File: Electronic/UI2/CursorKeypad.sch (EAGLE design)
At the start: 22 parts, among them IC1 74HCT14N

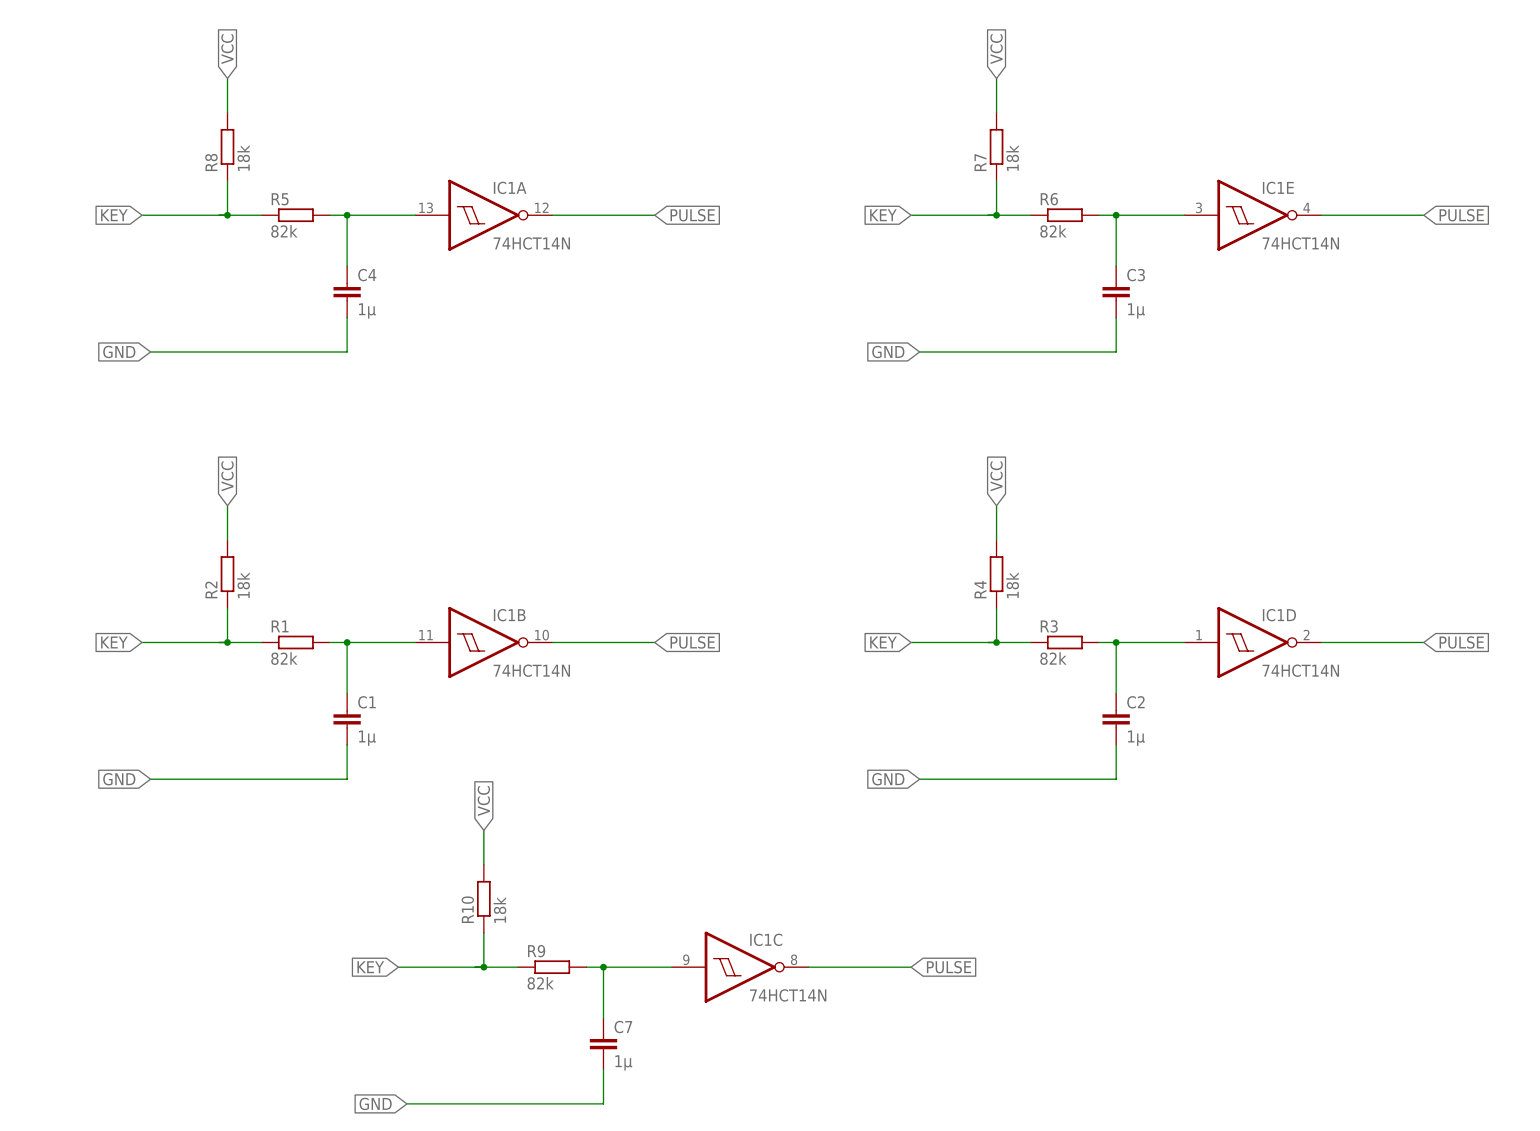
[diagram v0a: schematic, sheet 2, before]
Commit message: new UI
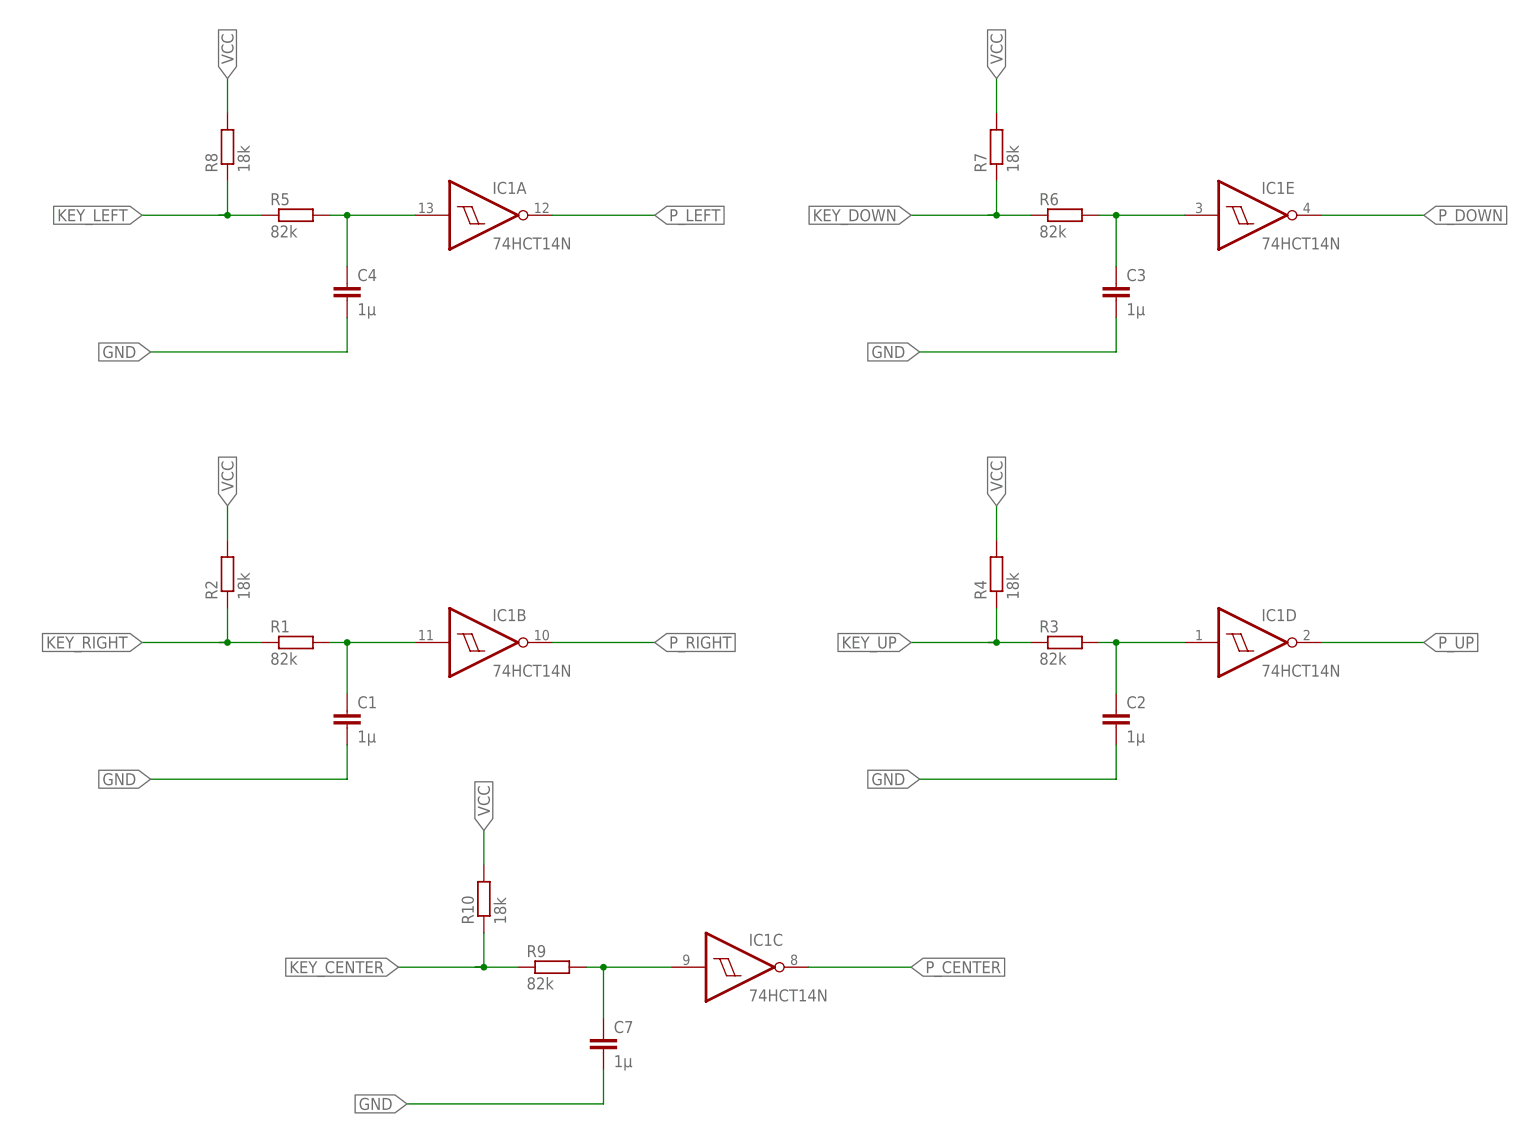
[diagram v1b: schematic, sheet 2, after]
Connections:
- removed net KEY: R1.1, R10.1, R2.1, R3.1, R4.1, R5.1, R6.1, R7.1, R8.1, R9.1
- removed net PULSE: IC1A.O, IC1B.O, IC1C.O, IC1D.O, IC1E.O
- new net P_CENTER: IC1C.O
- new net P_DOWN: IC1E.O
- new net P_LEFT: IC1A.O
- new net P_RIGHT: IC1B.O
- new net P_UP: IC1D.O
- net KEY_CENTER: now also R10.1, R9.1
- net KEY_DOWN: now also R6.1, R7.1
- net KEY_LEFT: now also R5.1, R8.1
- net KEY_RIGHT: now also R1.1, R2.1
- net KEY_UP: now also R3.1, R4.1
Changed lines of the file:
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@@
 </segment>
 </net>
-<net name="PULSE" class="0">
-<segment>
-<wire x1="91.44" y1="139.7" x2="106.68" y2="139.7" width="0.1524" layer="91"/>
-<label x="106.68" y="139.7" size="1.778" layer="95" xref="yes"/>
-<pinref part="IC1" gate="A" pin="O"/>
-</segment>
-<segment>
-<wire x1="91.44" y1="76.2" x2="106.68" y2="76.2" width="0.1524" layer="91"/>
-<label x="106.68" y="76.2" size="1.778" layer="95" xref="yes"/>
-<pinref part="IC1" gate="B" pin="O"/>
-</segment>
-<segment>
-<wire x1="205.74" y1="76.2" x2="220.98" y2="76.2" width="0.1524" layer="91"/>
-<label x="220.98" y="76.2" size="1.778" layer="95" xref="yes"/>
-<pinref part="IC1" gate="D" pin="O"/>
-</segment>
+<net name="P_DOWN" class="0">
 <segment>
 <wire x1="205.74" y1="139.7" x2="220.98" y2="139.7" width="0.1524" layer="91"/>
 <label x="220.98" y="139.7" size="1.778" layer="95" xref="yes"/>
 <pinref part="IC1" gate="E" pin="O"/>
-</segment>
-<segment>
-<wire x1="129.54" y1="27.94" x2="144.78" y2="27.94" width="0.1524" layer="91"/>
-<label x="144.78" y="27.94" size="1.778" layer="95" xref="yes"/>
-<pinref part="IC1" gate="C" pin="O"/>
 </segment>
 </net>
@@
 </segment>
 </net>
-<net name="KEY" class="0">
-<segment>
-<wire x1="43.18" y1="139.7" x2="30.48" y2="139.7" width="0.1524" layer="91"/>
-<wire x1="41.91" y1="139.7" x2="43.18" y2="139.7" width="0.1524" layer="91"/>
-<pinref part="R5" gate="G$1" pin="1"/>
-<pinref part="R8" gate="G$1" pin="1"/>
-<wire x1="43.18" y1="139.7" x2="48.26" y2="139.7" width="0.1524" layer="91"/>
-<wire x1="43.18" y1="144.78" x2="43.18" y2="139.7" width="0.1524" layer="91"/>
-<junction x="43.18" y="139.7"/>
-<label x="30.48" y="139.7" size="1.778" layer="95" rot="R180" xref="yes"/>
-</segment>
-<segment>
-<wire x1="43.18" y1="76.2" x2="30.48" y2="76.2" width="0.1524" layer="91"/>
-<wire x1="41.91" y1="76.2" x2="43.18" y2="76.2" width="0.1524" layer="91"/>
-<pinref part="R1" gate="G$1" pin="1"/>
-<pinref part="R2" gate="G$1" pin="1"/>
-<wire x1="43.18" y1="76.2" x2="48.26" y2="76.2" width="0.1524" layer="91"/>
-<wire x1="43.18" y1="81.28" x2="43.18" y2="76.2" width="0.1524" layer="91"/>
-<junction x="43.18" y="76.2"/>
-<label x="30.48" y="76.2" size="1.778" layer="95" rot="R180" xref="yes"/>
-</segment>
-<segment>
-<wire x1="157.48" y1="76.2" x2="144.78" y2="76.2" width="0.1524" layer="91"/>
-<wire x1="156.21" y1="76.2" x2="157.48" y2="76.2" width="0.1524" layer="91"/>
-<pinref part="R3" gate="G$1" pin="1"/>
-<pinref part="R4" gate="G$1" pin="1"/>
-<wire x1="157.48" y1="76.2" x2="162.56" y2="76.2" width="0.1524" layer="91"/>
-<wire x1="157.48" y1="81.28" x2="157.48" y2="76.2" width="0.1524" layer="91"/>
-<junction x="157.48" y="76.2"/>
-<label x="144.78" y="76.2" size="1.778" layer="95" rot="R180" xref="yes"/>
-</segment>
+<net name="KEY_DOWN" class="0">
 <segment>
 <wire x1="157.48" y1="139.7" x2="144.78" y2="139.7" width="0.1524" layer="91"/>
@@
 <junction x="157.48" y="139.7"/>
 <label x="144.78" y="139.7" size="1.778" layer="95" rot="R180" xref="yes"/>
-</segment>
-<segment>
-<wire x1="81.28" y1="27.94" x2="68.58" y2="27.94" width="0.1524" layer="91"/>
-<wire x1="80.01" y1="27.94" x2="81.28" y2="27.94" width="0.1524" layer="91"/>
-<pinref part="R9" gate="G$1" pin="1"/>
-<pinref part="R10" gate="G$1" pin="1"/>
-<wire x1="81.28" y1="27.94" x2="86.36" y2="27.94" width="0.1524" layer="91"/>
-<wire x1="81.28" y1="33.02" x2="81.28" y2="27.94" width="0.1524" layer="91"/>
-<junction x="81.28" y="27.94"/>
-<label x="68.58" y="27.94" size="1.778" layer="95" rot="R180" xref="yes"/>
 </segment>
 </net>
@@
 </segment>
 </net>
+<net name="KEY_LEFT" class="0">
+<segment>
+<wire x1="43.18" y1="139.7" x2="30.48" y2="139.7" width="0.1524" layer="91"/>
+<wire x1="41.91" y1="139.7" x2="43.18" y2="139.7" width="0.1524" layer="91"/>
+<pinref part="R5" gate="G$1" pin="1"/>
+<pinref part="R8" gate="G$1" pin="1"/>
+<wire x1="43.18" y1="139.7" x2="48.26" y2="139.7" width="0.1524" layer="91"/>
+<wire x1="43.18" y1="144.78" x2="43.18" y2="139.7" width="0.1524" layer="91"/>
+<junction x="43.18" y="139.7"/>
+<label x="30.48" y="139.7" size="1.778" layer="95" rot="R180" xref="yes"/>
+</segment>
+</net>
+<net name="KEY_RIGHT" class="0">
+<segment>
+<wire x1="43.18" y1="76.2" x2="30.48" y2="76.2" width="0.1524" layer="91"/>
+<wire x1="41.91" y1="76.2" x2="43.18" y2="76.2" width="0.1524" layer="91"/>
+<pinref part="R1" gate="G$1" pin="1"/>
+<pinref part="R2" gate="G$1" pin="1"/>
+<wire x1="43.18" y1="76.2" x2="48.26" y2="76.2" width="0.1524" layer="91"/>
+<wire x1="43.18" y1="81.28" x2="43.18" y2="76.2" width="0.1524" layer="91"/>
+<junction x="43.18" y="76.2"/>
+<label x="30.48" y="76.2" size="1.778" layer="95" rot="R180" xref="yes"/>
+</segment>
+</net>
+<net name="KEY_CENTER" class="0">
+<segment>
+<wire x1="81.28" y1="27.94" x2="68.58" y2="27.94" width="0.1524" layer="91"/>
+<wire x1="80.01" y1="27.94" x2="81.28" y2="27.94" width="0.1524" layer="91"/>
+<pinref part="R9" gate="G$1" pin="1"/>
+<pinref part="R10" gate="G$1" pin="1"/>
+<wire x1="81.28" y1="27.94" x2="86.36" y2="27.94" width="0.1524" layer="91"/>
+<wire x1="81.28" y1="33.02" x2="81.28" y2="27.94" width="0.1524" layer="91"/>
+<junction x="81.28" y="27.94"/>
+<label x="68.58" y="27.94" size="1.778" layer="95" rot="R180" xref="yes"/>
+</segment>
+</net>
+<net name="KEY_UP" class="0">
+<segment>
+<wire x1="157.48" y1="76.2" x2="144.78" y2="76.2" width="0.1524" layer="91"/>
+<wire x1="156.21" y1="76.2" x2="157.48" y2="76.2" width="0.1524" layer="91"/>
+<pinref part="R3" gate="G$1" pin="1"/>
+<pinref part="R4" gate="G$1" pin="1"/>
+<wire x1="157.48" y1="76.2" x2="162.56" y2="76.2" width="0.1524" layer="91"/>
+<wire x1="157.48" y1="81.28" x2="157.48" y2="76.2" width="0.1524" layer="91"/>
+<junction x="157.48" y="76.2"/>
+<label x="144.78" y="76.2" size="1.778" layer="95" rot="R180" xref="yes"/>
+</segment>
+</net>
+<net name="P_LEFT" class="0">
+<segment>
+<wire x1="91.44" y1="139.7" x2="106.68" y2="139.7" width="0.1524" layer="91"/>
+<label x="106.68" y="139.7" size="1.778" layer="95" xref="yes"/>
+<pinref part="IC1" gate="A" pin="O"/>
+</segment>
+</net>
+<net name="P_RIGHT" class="0">
+<segment>
+<wire x1="91.44" y1="76.2" x2="106.68" y2="76.2" width="0.1524" layer="91"/>
+<label x="106.68" y="76.2" size="1.778" layer="95" xref="yes"/>
+<pinref part="IC1" gate="B" pin="O"/>
+</segment>
+</net>
+<net name="P_CENTER" class="0">
+<segment>
+<wire x1="129.54" y1="27.94" x2="144.78" y2="27.94" width="0.1524" layer="91"/>
+<label x="144.78" y="27.94" size="1.778" layer="95" xref="yes"/>
+<pinref part="IC1" gate="C" pin="O"/>
+</segment>
+</net>
+<net name="P_UP" class="0">
+<segment>
+<wire x1="205.74" y1="76.2" x2="220.98" y2="76.2" width="0.1524" layer="91"/>
+<label x="220.98" y="76.2" size="1.778" layer="95" xref="yes"/>
+<pinref part="IC1" gate="D" pin="O"/>
+</segment>
+</net>
